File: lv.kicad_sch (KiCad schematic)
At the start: 8 parts, among them J10 CAN_NANO_01x05, J11 CAN_NANO_01x05, J8 CarLVPowerConnector, J9 CAN_DEBUG_NANO_01x04

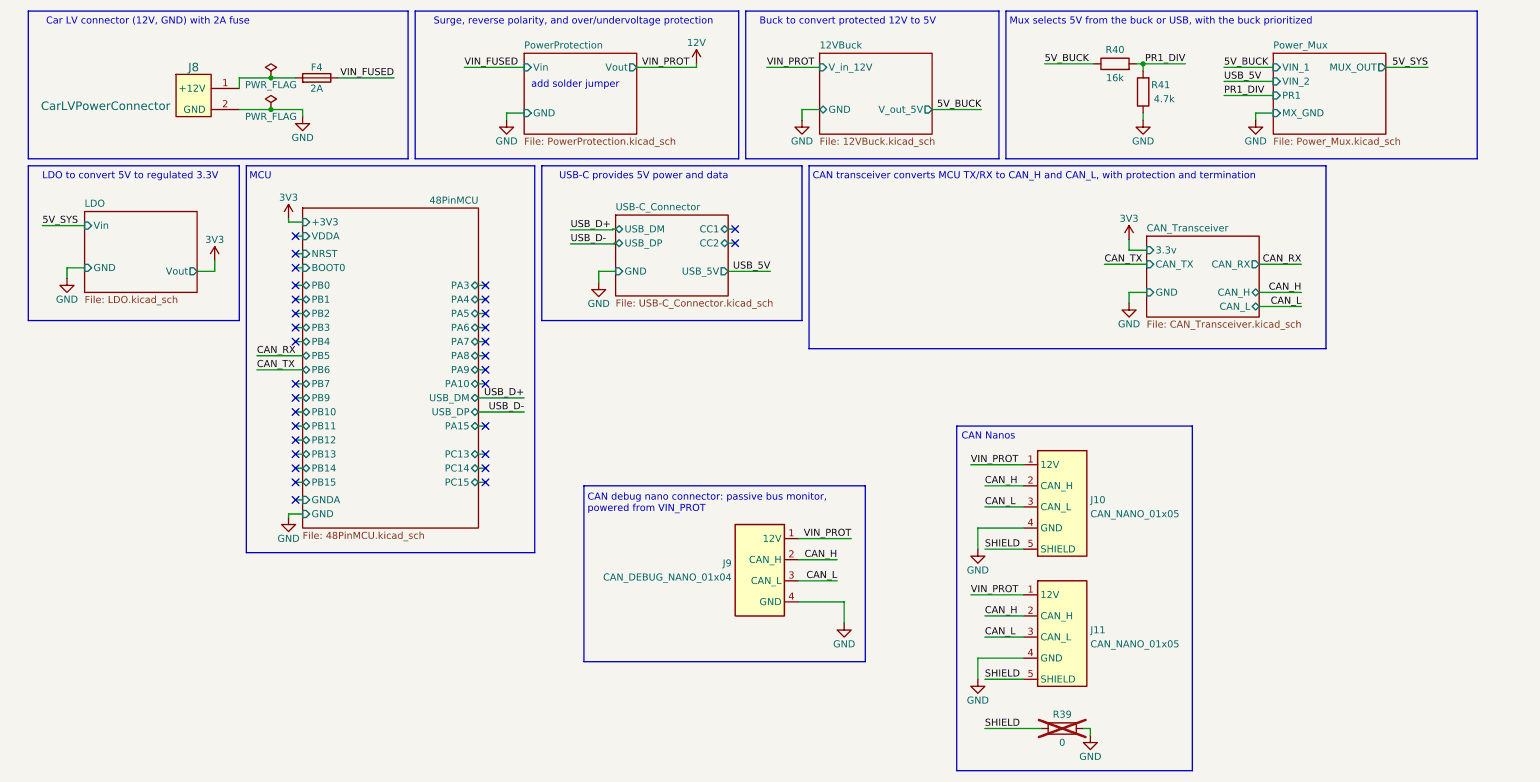
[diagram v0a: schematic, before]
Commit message: reorganized lv
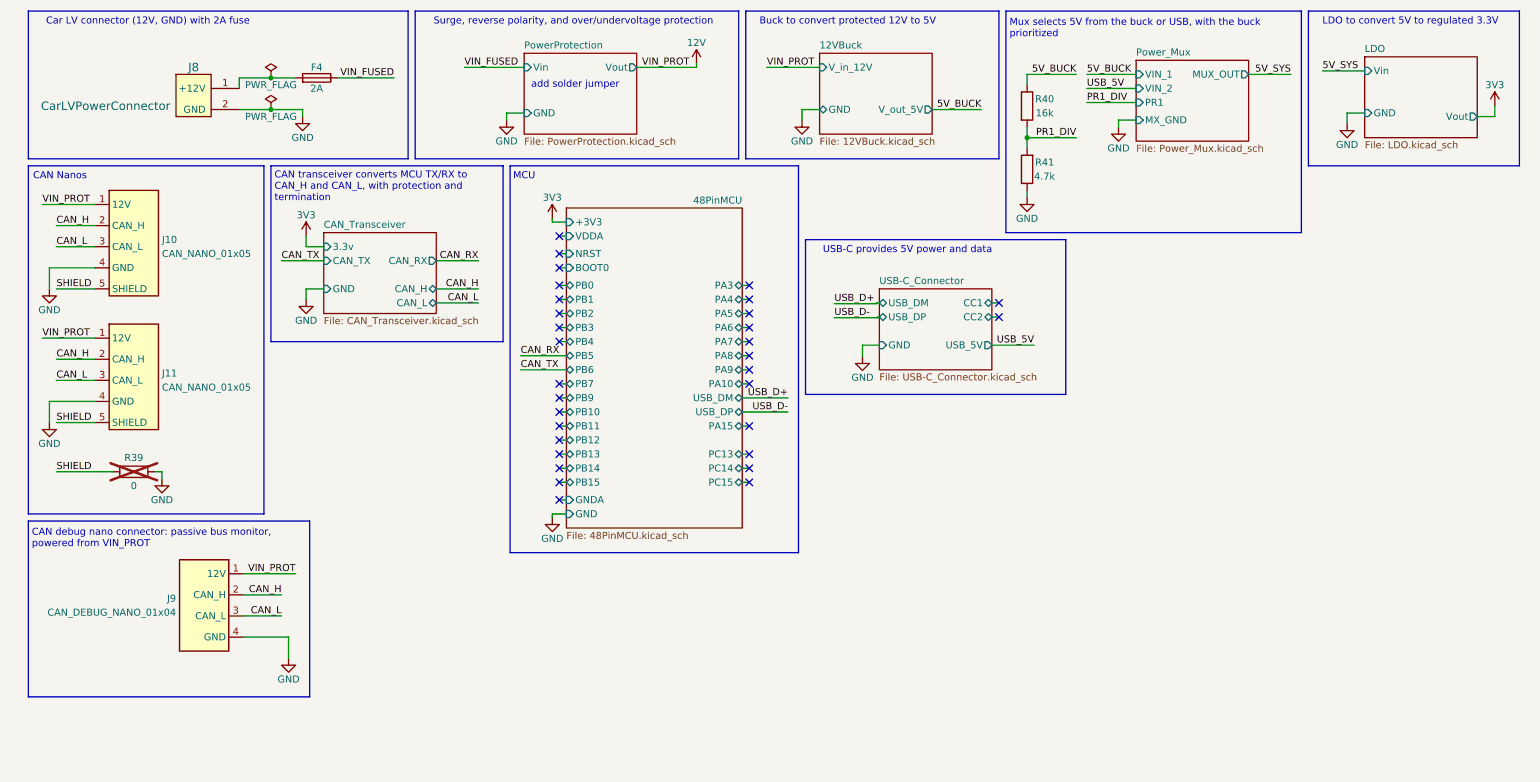
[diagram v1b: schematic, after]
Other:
- moved on the sheet: J10, J11, J9, R39, R40, R41
